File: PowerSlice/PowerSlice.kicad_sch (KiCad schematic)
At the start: 25 parts, among them J1 Conn_01x08_Pin, J2 Barrel_Jack, J3 Screw_Terminal_01x02, SW1 SW_ESTOP, U1 PTH08080WAD, U2 PTH08080WAD, U3 INA214BIDCKR, U4 INA214BIDCKR, U5 INA214BIDCKR, U6 NUCLEO-F303K8

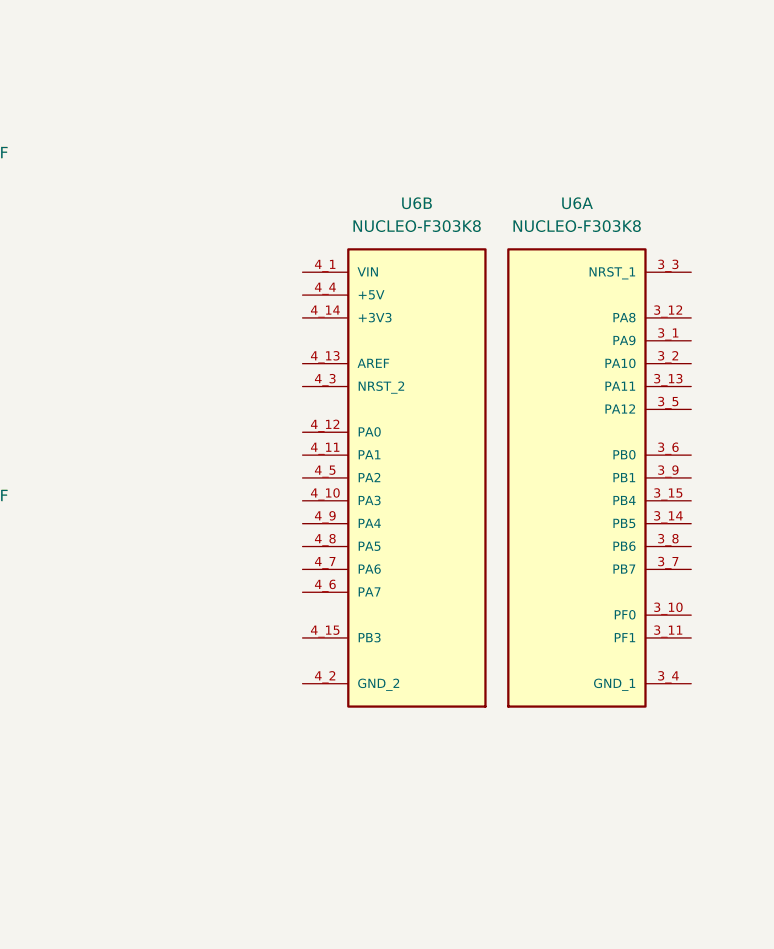
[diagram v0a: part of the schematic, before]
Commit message: Update PowerSlice.kicad_sch
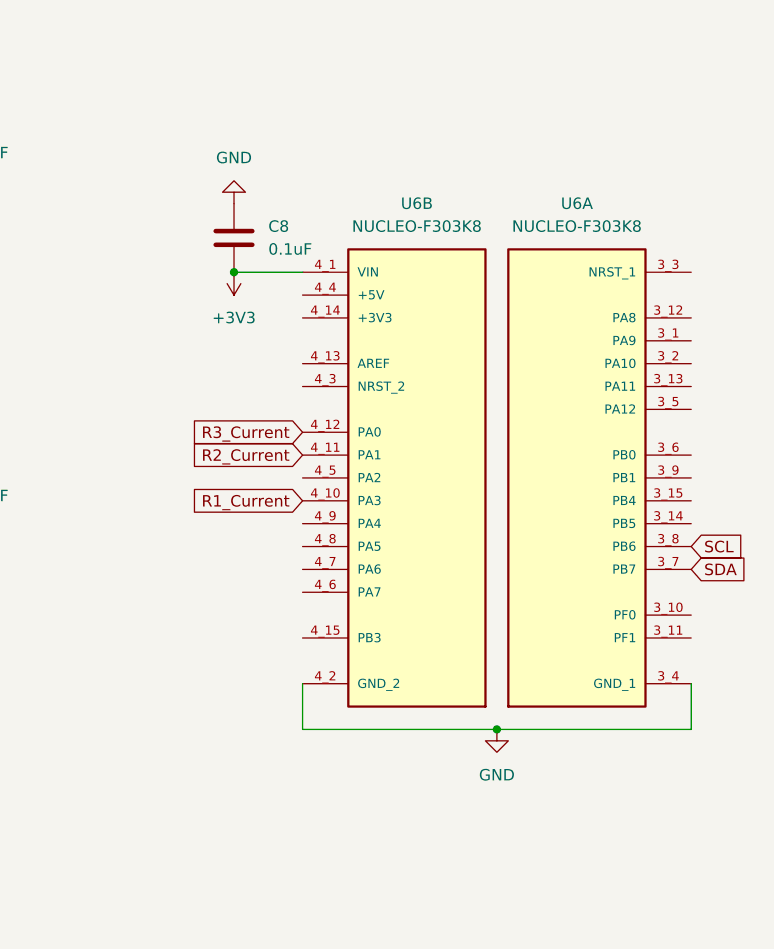
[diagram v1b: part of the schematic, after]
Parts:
- added C8: 0.1uF, symbol Device:C
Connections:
- net +3V3: now also U6.4_1 (VIN), C8.2
- net GND: now also U6.3_4 (GND_1), U6.4_2 (GND_2), C8.1
- net R1_Current: now also U6.4_10 (PA3)
- net R2_Current: now also U6.4_11 (PA1)
- net R3_Current: now also U6.4_12 (PA0)
- net SCL: now also U6.3_8 (PB6)
- net SDA: now also U6.3_7 (PB7)

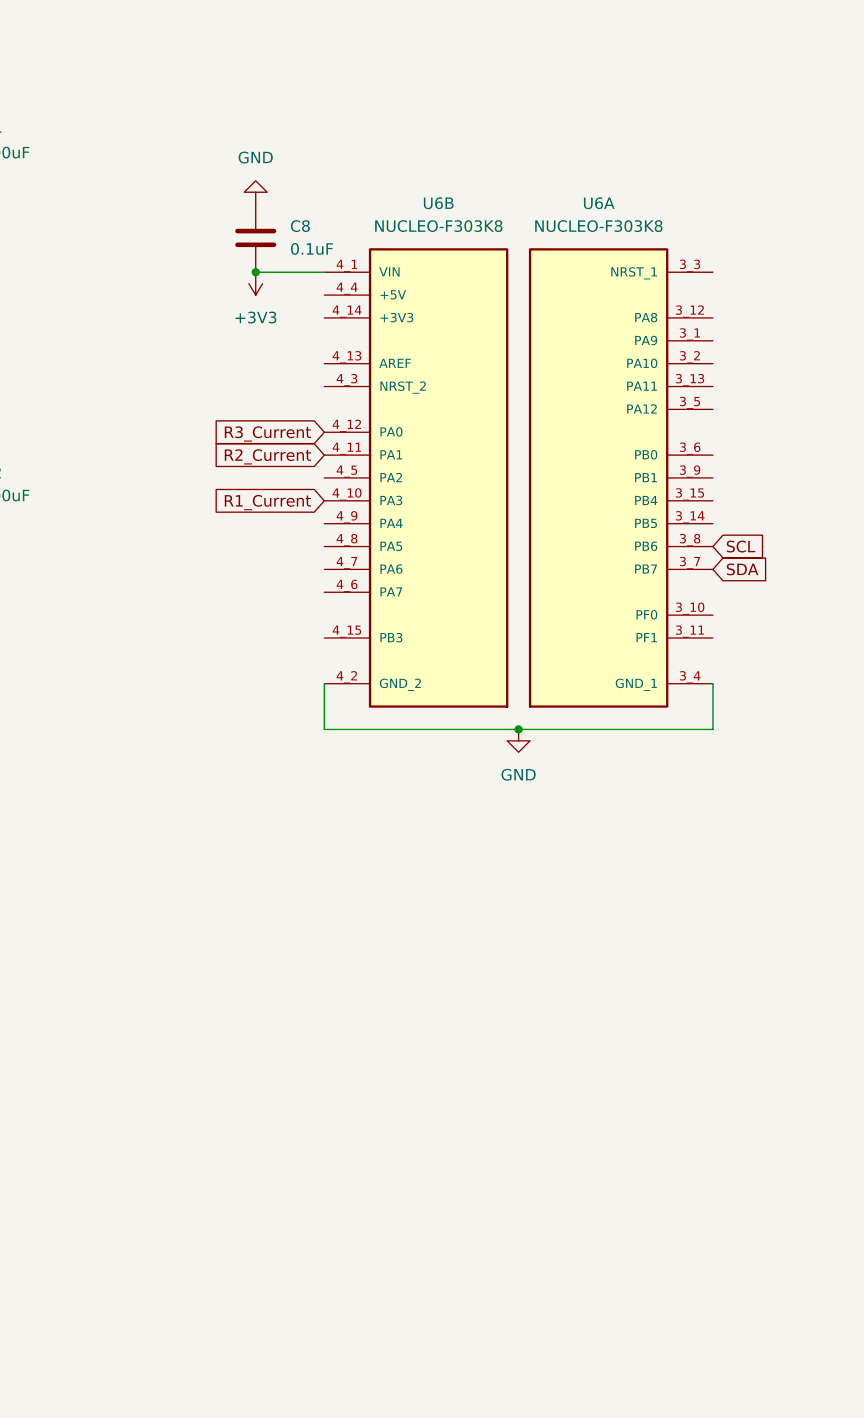
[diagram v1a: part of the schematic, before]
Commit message: finished preliminary schematic
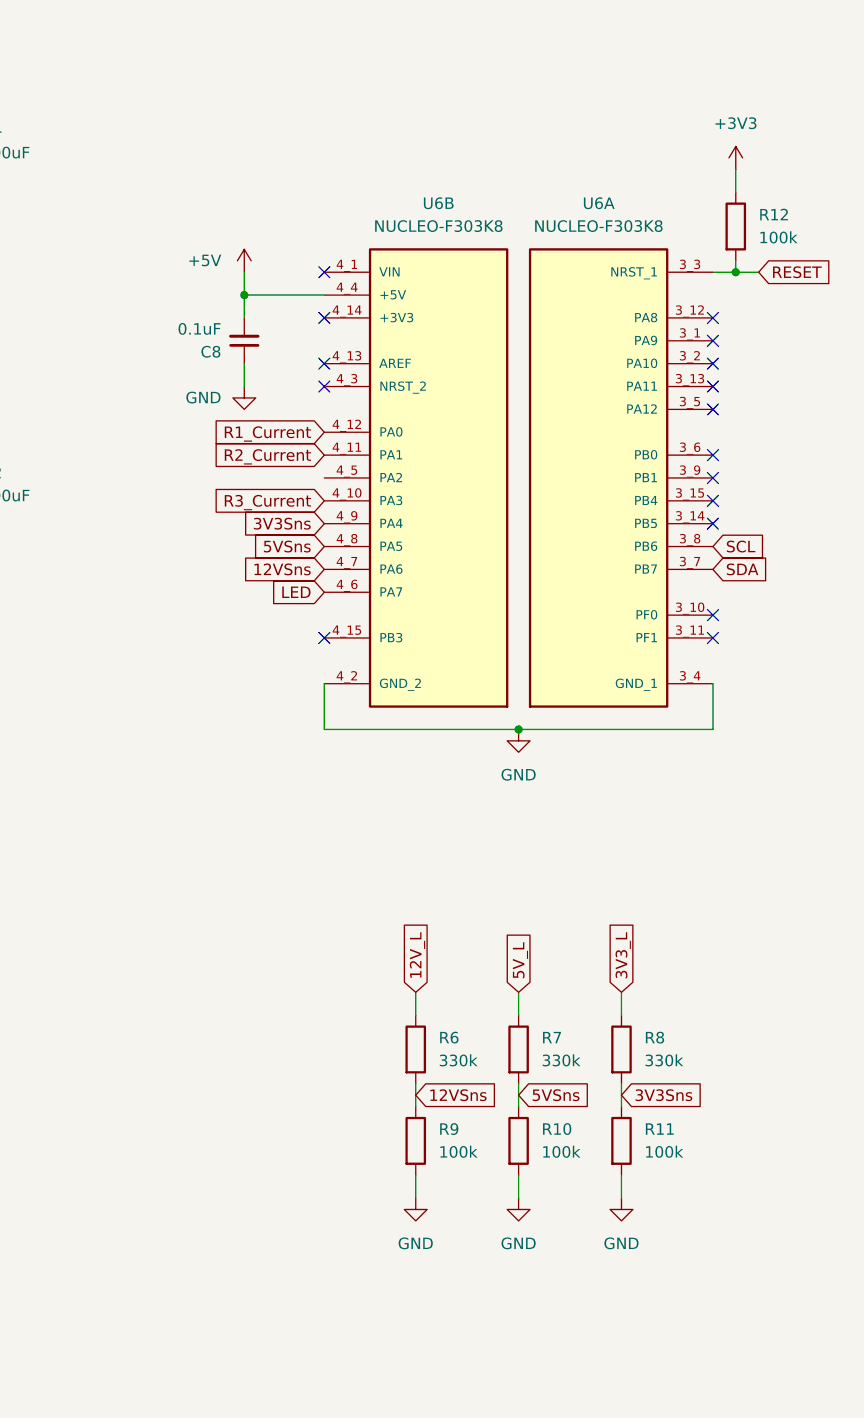
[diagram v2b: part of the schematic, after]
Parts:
- removed C8: 0.1uF, symbol Device:C
- added C8: 0.1uF, symbol Device:C_Small
- added R10, R11, R12, R9: 100k, symbol Device:R
- added R6, R7, R8: 330k, symbol Device:R
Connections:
- net +3V3: now also R12.1; no longer U6.4_1 (VIN)
- net +5V: now also U6.4_4 (+5V), C8.2
- net 12V_L: now also R6.1
- net 3V3_L: now also R8.1
- net 5V_L: now also R7.1
- net GND: now also C8.1, R10.2, R11.2, R9.2
- net LED: now also U6.4_6 (PA7)
- net R1_Current: now also U6.4_12 (PA0); no longer U6.4_10 (PA3)
- net R3_Current: now also U6.4_10 (PA3); no longer U6.4_12 (PA0)
- net RESET: now also U6.3_3 (NRST_1), R12.2
- net 12VSns: now reaches U6.4_7 (PA6)
- net 12VSns: now also R6.2, R9.1
- net 5VSns: now reaches U6.4_8 (PA5)
- net 5VSns: now also R10.1, R7.2
- net 3V3Sns: now reaches U6.4_9 (PA4)
- net 3V3Sns: now also R11.1, R8.2
- no-connect marks 2 -> 18
